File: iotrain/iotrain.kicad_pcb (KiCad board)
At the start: 2 copper layers, 21.2 x 14 mm, 68 parts, among them J1 12V, J10 X2, J11 SCL, J12 SDA, J13 GND, J14 3V3, J15 GND, J16 USB_B_Micro, J2 PROG ESP, J3 AC1, J4 AC1, J5 LSP, J6 LSP, J7 M1, J8 M2, J9 X1, Q1 TPM2008 EP3-A, Q2 TPM2008 EP3-A, SW1 Reset, SW2 Boot, U2 MAX98357A_WLP_Package, U3 TPS82130, U4 ESP32-C6FH4, U6 IPS_160_40_10P, U7 DRV8876RGT, Y1 40MHz

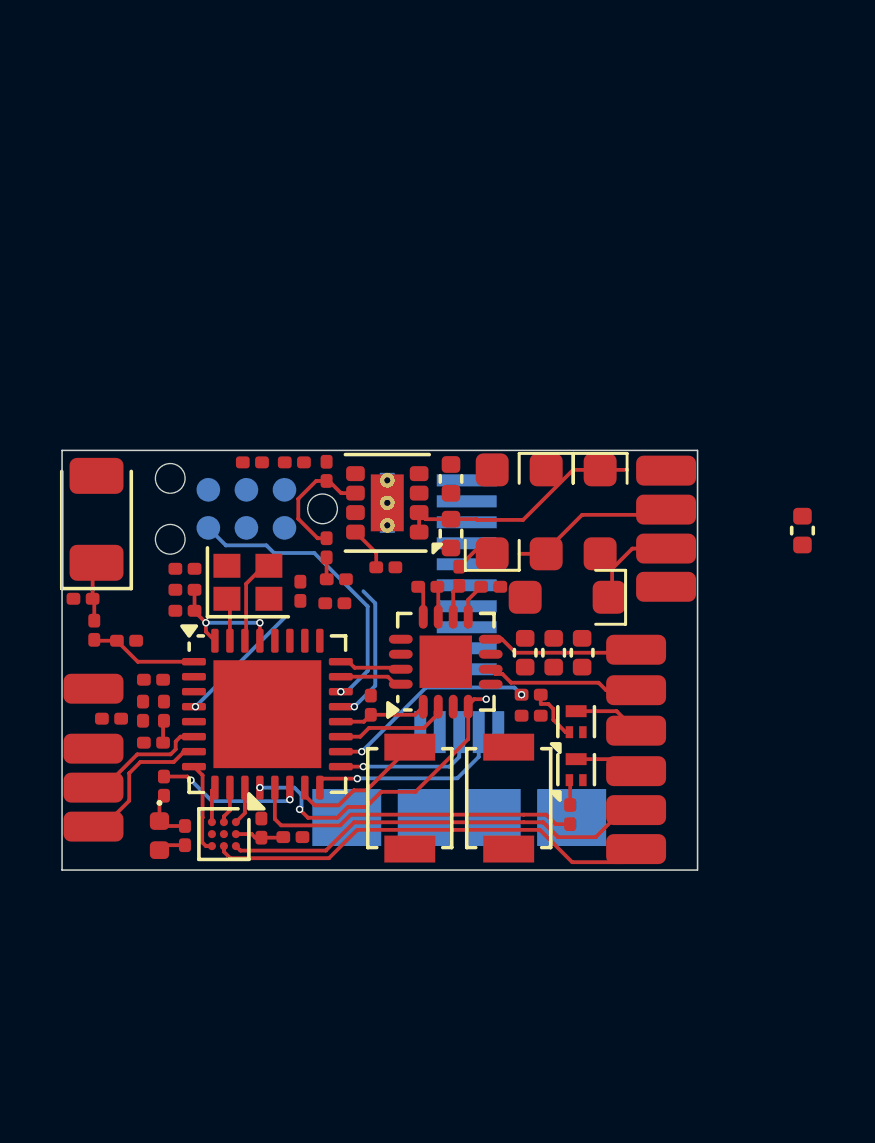
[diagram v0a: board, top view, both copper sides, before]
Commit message: Make it smaller
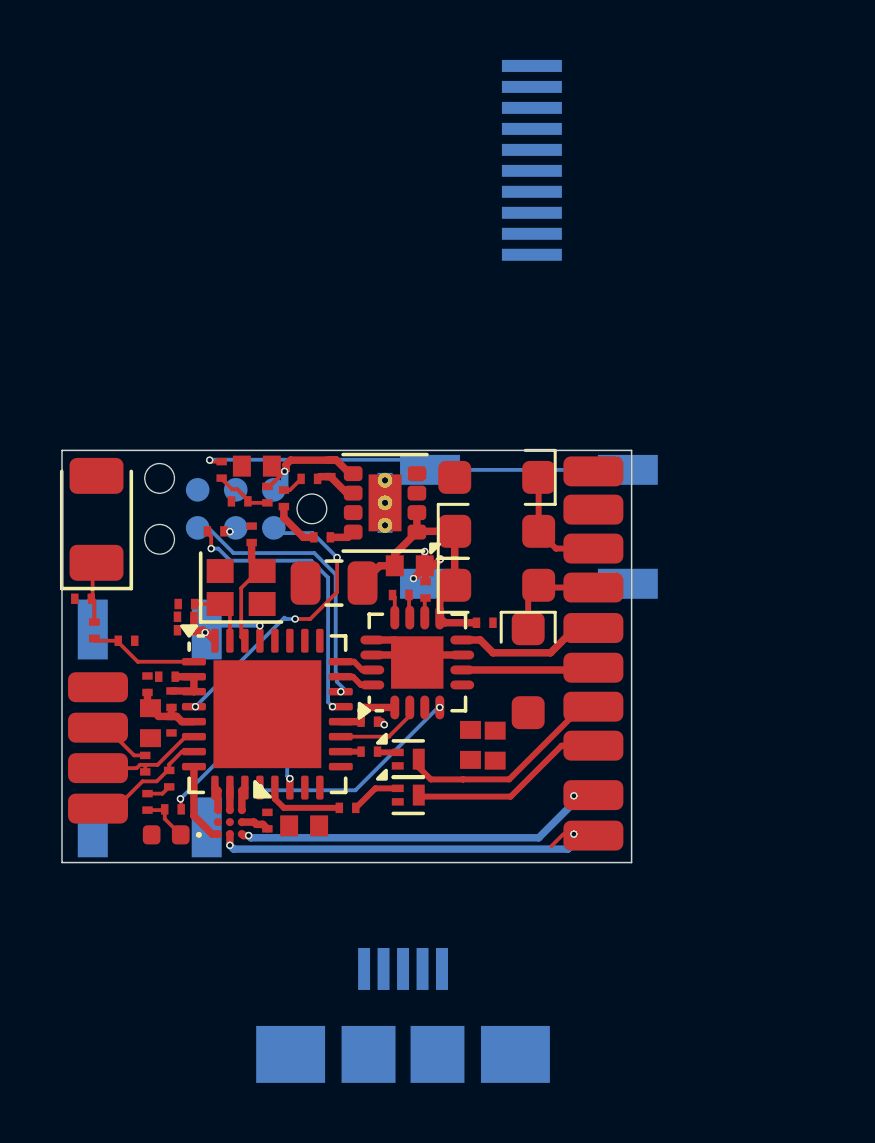
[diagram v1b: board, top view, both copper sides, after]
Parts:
- removed C13: 10u/20V, Capacitor_SMD:C_0402_1005Metric
- added R11: 1k, liebler_PASSIVES:SMD0201, F.Cu at (126.9, 63.1)
- added R12: 1k, liebler_PASSIVES:SMD0201, F.Cu at (127.7, 63.6)
- C1, C10, C14, C16, C19, C2, C21, C25, C26, C3, C4, C5, C6, C7, C8, C9: footprint Capacitor_SMD:C_0201_0603Metric -> liebler_PASSIVES:SMD0201
- C11: footprint Capacitor_SMD:C_0402_1005Metric -> Capacitor_SMD:C_0805_2012Metric
- C12, C18: footprint Capacitor_SMD:C_0201_0603Metric -> liebler_PASSIVES:SMD0402
- C15, C17, C20, C22: footprint Capacitor_SMD:C_0402_1005Metric -> liebler_PASSIVES:SMD0402
- L1, L2: footprint Inductor_SMD:L_0201_0603Metric -> liebler_PASSIVES:SMD0201
- R1, R10, R2, R3, R4, R5, R6, R7, R8, R9: footprint Resistor_SMD:R_0201_0603Metric -> liebler_PASSIVES:SMD0201
- SW1, SW2: footprint Button_Switch_SMD:SW_SPST_B3U-1000P -> liebler_MECH:SW_SPST_TL3342_smaller_handsolder; moved to B.Cu
- moved U6 14.0 mm to (139.8, 43.0)
- moved R7 13.2 mm to (129.4, 53.3), turned to -90 degrees
- moved C22 12.5 mm to (138.6, 62.5)
- moved SW1 9.08 mm to (139.7, 55.2), turned to 0 degrees
- moved SW2 8.98 mm to (127.0, 61.9), turned to -90 degrees
- moved J16 8.12 mm to (135.5, 71.5)
- moved C11 7.69 mm to (133.2, 57.1), turned to 180 degrees
- moved R4 7.43 mm to (133.6, 64.6), turned to 0 degrees
- moved C17 6.49 mm to (130.6, 53.2), turned to 180 degrees
- moved Q2 5.74 mm to (135.7, 63.0), turned to 0 degrees
- moved R9 5.72 mm to (134.3, 62.7)
- moved Q1 5.66 mm to (135.7, 64.2), turned to 0 degrees
- moved D5 5.43 mm to (139.7, 60.0), turned to -90 degrees
- moved R1 4.64 mm to (129.2, 55.4), turned to 0 degrees
- moved D3 4.64 mm to (138.6, 53.5)
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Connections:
- C21 pad 1: PROG_EN -> CHIP_EN
- R5 pad 1: unconnected-(R5-Pad1) -> GND
- R7 pad 2: PROG_EN -> CHIP_EN
- R8 pad 1: PROG_EN -> CHIP_EN
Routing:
- net Net-(R7-Pad1): track 0.00 -> 14.4 mm, vias 0 -> 1
- net T1: track 11.3 -> 2.65 mm
- net GND: track 0.85 -> 9.14 mm, vias 0 -> 4
- net CHIP_EN: track 4.25 -> 12.0 mm, vias 1 -> 3
- net Net-(J16-D-): track 6.74 -> 0.00 mm, vias 1 -> 0
- net T2: track 7.01 -> 0.67 mm, vias 2 -> 0
- net +3V3: track 10.6 -> 16.5 mm, vias 2 -> 3
- net /X2: track 2.27 -> 7.27 mm
- net Net-(J16-D+): track 4.91 -> 0.00 mm, vias 1 -> 0
- net PROG_IO9: track 4.70 -> 0.00 mm
- net Net-(U4-U0TXD/GPIO16/FSPICS0): track 4.76 -> 9.39 mm, vias 1 -> 2
- net /X1: track 2.17 -> 6.55 mm
- net MOT_IPROPRI: track 10.6 -> 7.21 mm, vias 3 -> 2
- net Net-(U3-FB): track 4.20 -> 1.45 mm
- net /LSPP: track 14.4 -> 12.0 mm, vias 0 -> 2
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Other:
- board size 21.2 x 14 mm -> 19 x 13.8 mm
